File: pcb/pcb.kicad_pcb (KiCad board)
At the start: 4 copper layers, 60 x 60 mm, 112 parts, among them X1 USB_C_Receptacle_USB2.0, X2 Bat-Conn, X3 NTC, X4 UART, X5 SWD, Y1 32MHz, Y2 32.768k

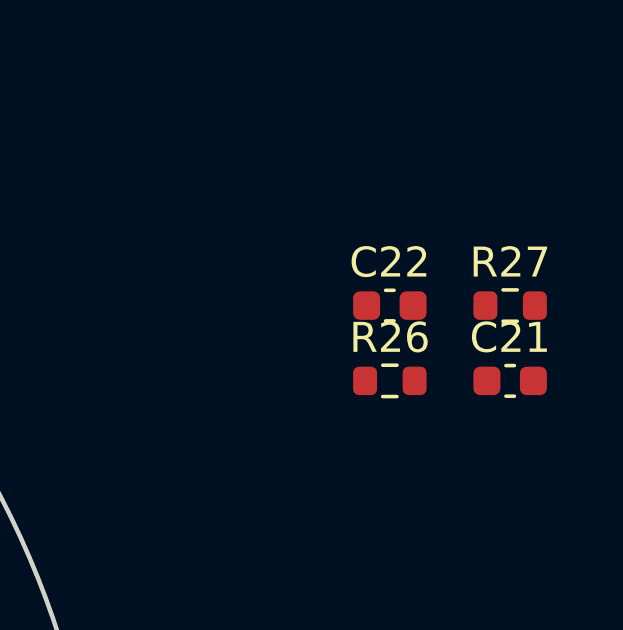
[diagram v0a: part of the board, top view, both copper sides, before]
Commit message: edit gitignore
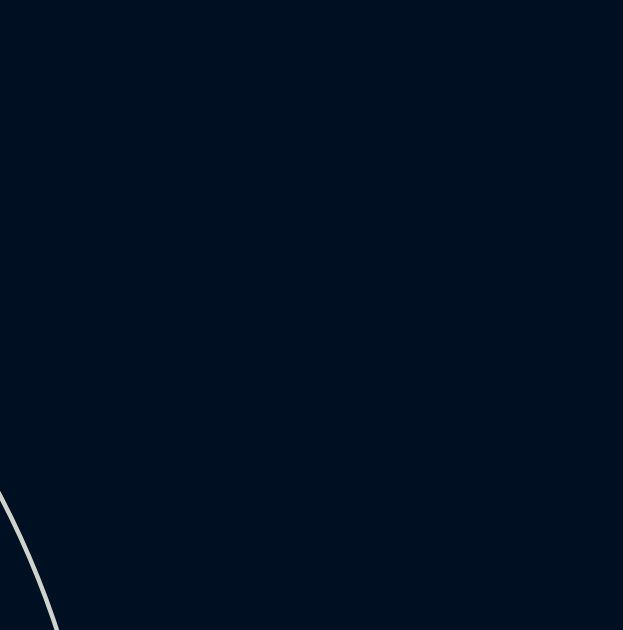
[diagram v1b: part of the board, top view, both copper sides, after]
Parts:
- removed C21: 100n, Capacitor_SMD:C_0603_1608Metric
- removed C22: 56p, Capacitor_SMD:C_0603_1608Metric
- removed R26: 1Meg, Resistor_SMD:R_0603_1608Metric
- removed R27: 324k, Resistor_SMD:R_0603_1608Metric
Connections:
- V4 pad 12: DCDC-FB -> 3.3V
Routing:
- net BAT_PROT-: track 258.7 -> 137.3 mm, vias 62 -> 55
- net Ring0_10: track 0.00 -> 51.4 mm, vias 0 -> 2
- net unconnected-(V33-Pad22): track 43.2 -> 0.00 mm, vias 1 -> 0
- net Ring1_6: track 0.00 -> 43.2 mm, vias 0 -> 1
- net Ring0_9: track 44.8 -> 81.7 mm, vias 1 -> 2
- net Ring0_5: track 48.8 -> 85.4 mm, vias 3 -> 4
- net Ring1_11: track 19.3 -> 0.00 mm, vias 1 -> 0
- net BAT_SENS: track 40.4 -> 25.1 mm, vias 5 -> 3
- net RXD: track 18.1 -> 33.4 mm, vias 2 -> 4
- net 3.3V: track 119.7 -> 128.9 mm
- net Ring1_1: track 5.89 -> 12.5 mm, vias 1 -> 5

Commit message: Revert "edit gitignore"
This reverts commit 7d0c4b0df1450372f941e83b064acac36d25e600.
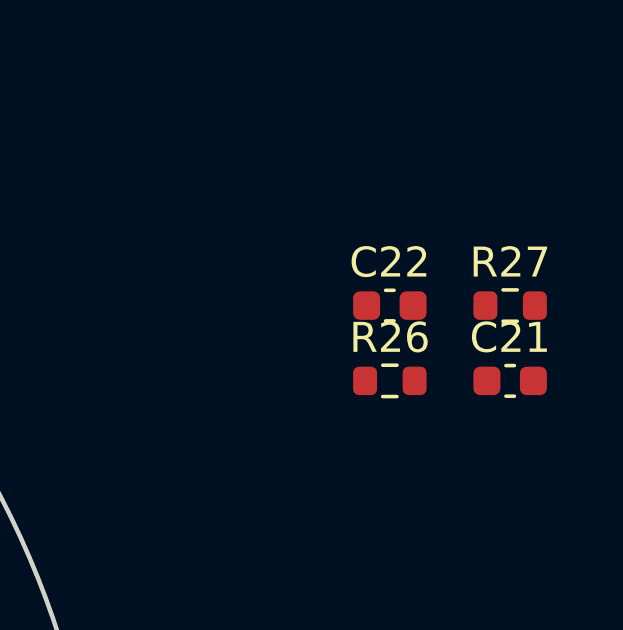
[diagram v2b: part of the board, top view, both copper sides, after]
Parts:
- added C21: 100n, Capacitor_SMD:C_0603_1608Metric, F.Cu at (193.6, 82.3)
- added C22: 56p, Capacitor_SMD:C_0603_1608Metric, F.Cu at (189.6, 79.8)
- added R26: 1Meg, Resistor_SMD:R_0603_1608Metric, F.Cu at (189.6, 82.3)
- added R27: 324k, Resistor_SMD:R_0603_1608Metric, F.Cu at (193.6, 79.8)
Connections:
- V4 pad 12: 3.3V -> DCDC-FB
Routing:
- net BAT_PROT-: track 137.3 -> 258.7 mm, vias 55 -> 62
- net Ring0_10: track 51.4 -> 0.00 mm, vias 2 -> 0
- net unconnected-(V33-Pad22): track 0.00 -> 43.2 mm, vias 0 -> 1
- net Ring1_6: track 43.2 -> 0.00 mm, vias 1 -> 0
- net Ring0_9: track 81.7 -> 44.8 mm, vias 2 -> 1
- net Ring0_5: track 85.4 -> 48.8 mm, vias 4 -> 3
- net Ring1_11: track 0.00 -> 19.3 mm, vias 0 -> 1
- net BAT_SENS: track 25.1 -> 40.4 mm, vias 3 -> 5
- net RXD: track 33.4 -> 18.1 mm, vias 4 -> 2
- net 3.3V: track 128.9 -> 119.7 mm
- net Ring1_1: track 12.5 -> 5.89 mm, vias 5 -> 1
